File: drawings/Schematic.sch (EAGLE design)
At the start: 15 parts

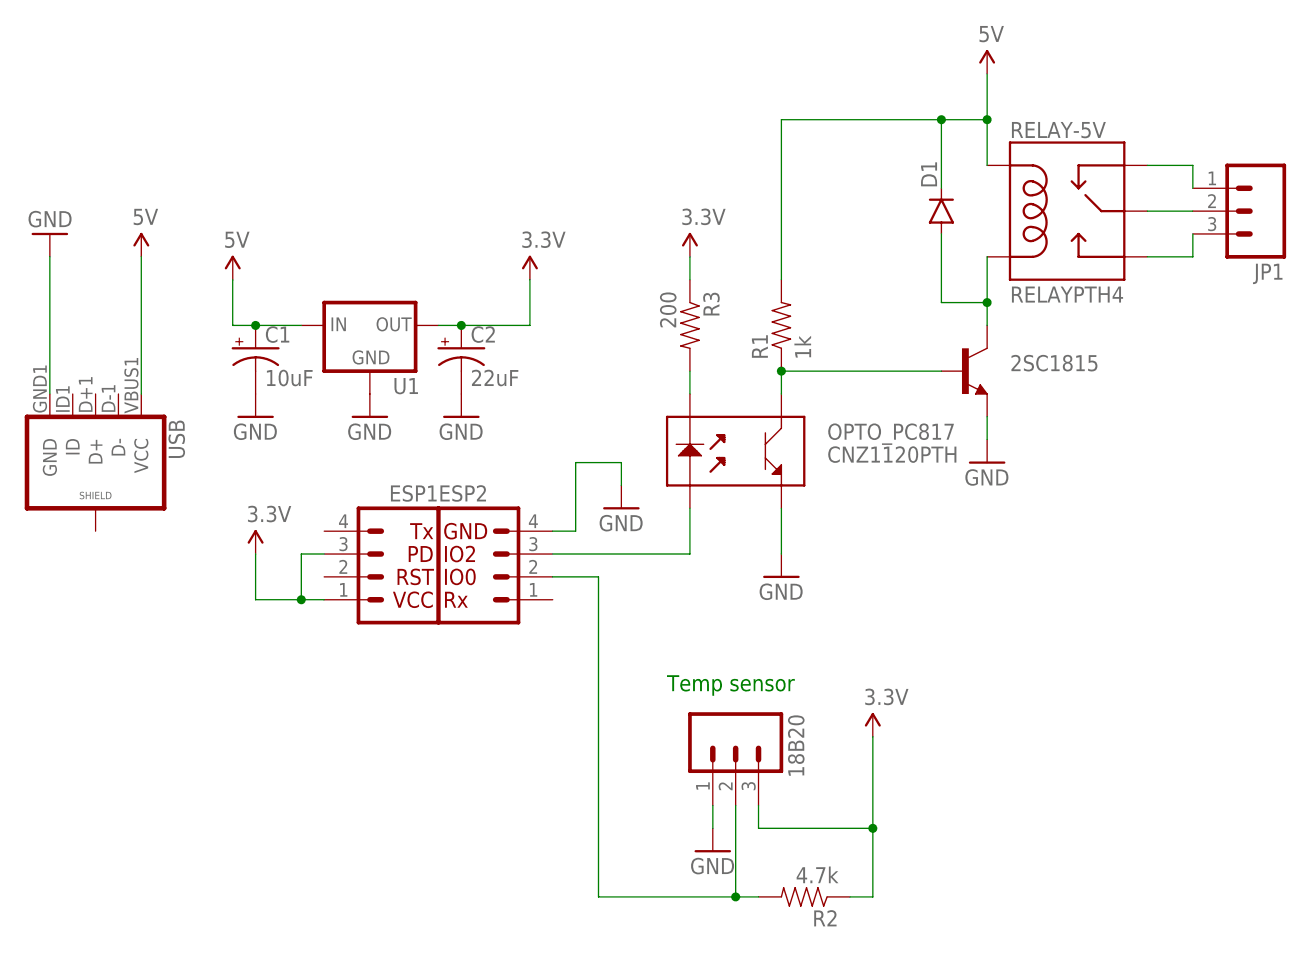
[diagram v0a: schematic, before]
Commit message: revise drawings
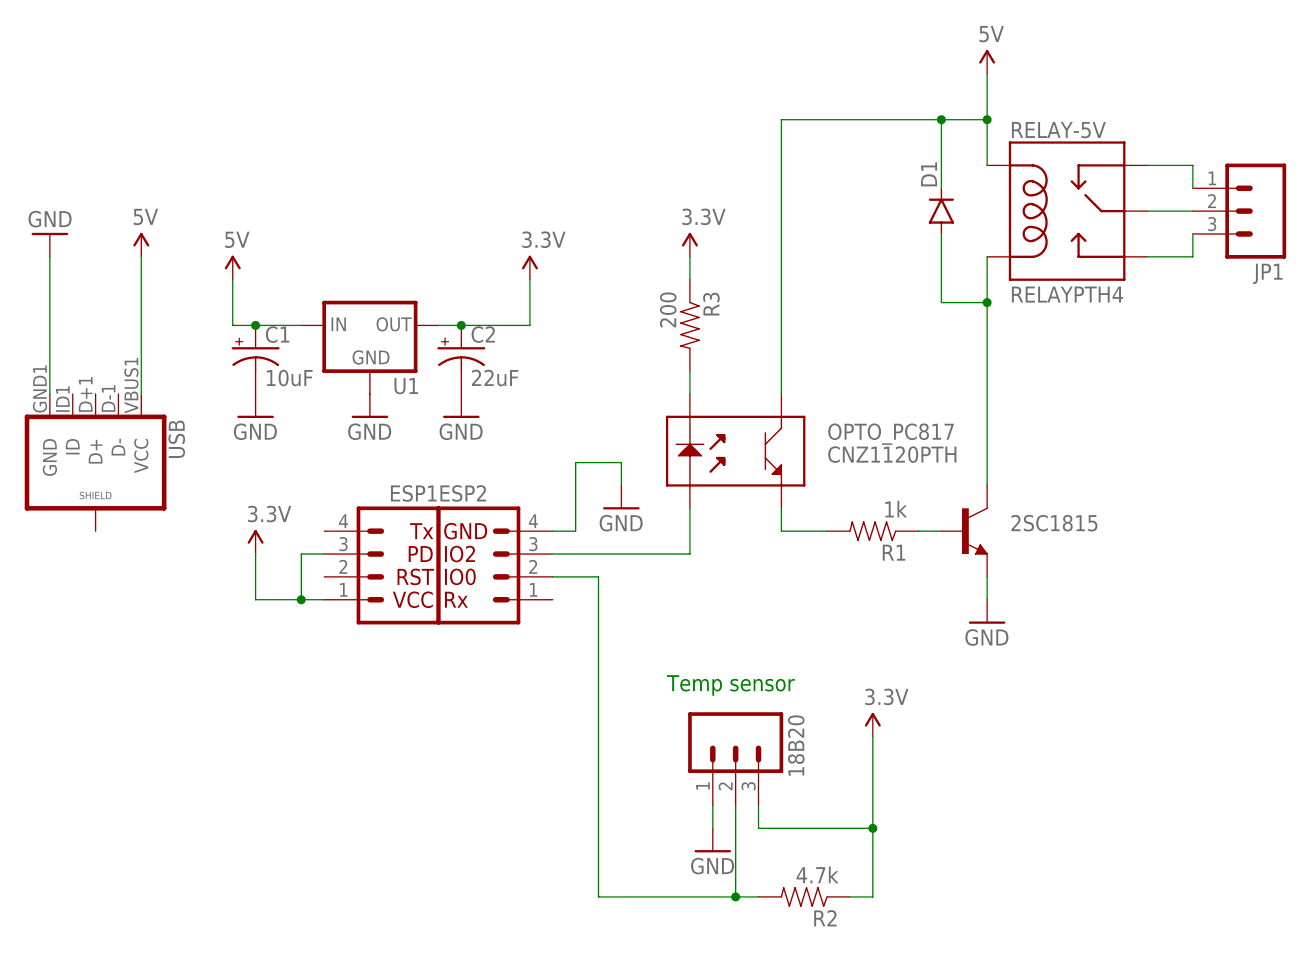
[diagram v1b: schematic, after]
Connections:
- new net N$9: 2SC1815.B, R1.1
- net 5V: now also OPTO_PC817.3; no longer R1.2
- net GND: no longer OPTO_PC817.4
- net N$1: now also OPTO_PC817.4, R1.2; no longer 2SC1815.B, OPTO_PC817.3, R1.1
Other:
- moved on the sheet: 2SC1815, R1
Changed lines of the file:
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@@
 <part name="R3" library="SparkFun-Resistors" deviceset="10KOHM-1/4W5%(PTH)" device="" value="200"/>
 <part name="SUPPLY8" library="SparkFun-Aesthetics" deviceset="3.3V" device=""/>
-<part name="GND7" library="SparkFun-Aesthetics" deviceset="GND" device=""/>
 <part name="JP1" library="ESP8266" deviceset="M03" device="1X03_NO_SILK"/>
 </parts>
@@
 <instance part="SUPPLY1" gate="G$1" x="17.78" y="38.1"/>
 <instance part="GND4" gate="1" x="58.42" y="43.18"/>
-<instance part="R1" gate="G$1" x="76.2" y="63.5" rot="R90"/>
-<instance part="2SC1815" gate="G$1" x="96.52" y="58.42"/>
+<instance part="R1" gate="G$1" x="86.36" y="40.64" rot="R180"/>
+<instance part="2SC1815" gate="G$1" x="96.52" y="40.64"/>
 <instance part="RELAY-5V" gate="G$1" x="109.22" y="76.2"/>
 <instance part="SUPPLY4" gate="G$1" x="99.06" y="91.44"/>
-<instance part="GND5" gate="1" x="99.06" y="48.26"/>
+<instance part="GND5" gate="1" x="99.06" y="30.48"/>
 <instance part="18B20" gate="G$1" x="71.12" y="17.78" rot="R270"/>
 <instance part="GND6" gate="1" x="68.58" y="5.08"/>
@@
 <instance part="R3" gate="G$1" x="66.04" y="63.5" rot="R270"/>
 <instance part="SUPPLY8" gate="G$1" x="66.04" y="71.12"/>
-<instance part="GND7" gate="1" x="76.2" y="35.56"/>
 <instance part="JP1" gate="G$1" x="129.54" y="76.2" rot="R180"/>
 </instances>
@@
 <wire x1="93.98" y1="86.36" x2="76.2" y2="86.36" width="0.1524" layer="91"/>
 <junction x="93.98" y="86.36"/>
-<pinref part="R1" gate="G$1" pin="2"/>
-<wire x1="76.2" y1="86.36" x2="76.2" y2="68.58" width="0.1524" layer="91"/>
+<pinref part="OPTO_PC817" gate="G$1" pin="3"/>
+<wire x1="76.2" y1="86.36" x2="76.2" y2="55.88" width="0.1524" layer="91"/>
 </segment>
 <segment>
@@
 </segment>
 <segment>
-<pinref part="2SC1815" gate="G$1" pin="E"/>
-<pinref part="GND5" gate="1" pin="GND"/>
-<wire x1="99.06" y1="53.34" x2="99.06" y2="50.8" width="0.1524" layer="91"/>
-</segment>
-<segment>
 <pinref part="18B20" gate="G$1" pin="1"/>
 <pinref part="GND6" gate="1" pin="GND"/>
@@
 </segment>
 <segment>
-<pinref part="OPTO_PC817" gate="G$1" pin="4"/>
-<pinref part="GND7" gate="1" pin="GND"/>
-<wire x1="76.2" y1="43.18" x2="76.2" y2="38.1" width="0.1524" layer="91"/>
-</segment>
-</net>
-<net name="N$1" class="0">
-<segment>
-<pinref part="R1" gate="G$1" pin="1"/>
-<pinref part="2SC1815" gate="G$1" pin="B"/>
-<wire x1="76.2" y1="58.42" x2="93.98" y2="58.42" width="0.1524" layer="91"/>
-<junction x="76.2" y="58.42"/>
-<pinref part="OPTO_PC817" gate="G$1" pin="3"/>
-<wire x1="76.2" y1="58.42" x2="76.2" y2="55.88" width="0.1524" layer="91"/>
+<pinref part="2SC1815" gate="G$1" pin="E"/>
+<pinref part="GND5" gate="1" pin="GND"/>
+<wire x1="99.06" y1="35.56" x2="99.06" y2="33.02" width="0.1524" layer="91"/>
 </segment>
 </net>
@@
 <wire x1="99.06" y1="71.12" x2="99.06" y2="66.04" width="0.1524" layer="91"/>
 <pinref part="D1" gate="G$1" pin="A"/>
-<wire x1="99.06" y1="66.04" x2="99.06" y2="63.5" width="0.1524" layer="91"/>
+<wire x1="99.06" y1="66.04" x2="99.06" y2="45.72" width="0.1524" layer="91"/>
 <wire x1="93.98" y1="73.66" x2="93.98" y2="66.04" width="0.1524" layer="91"/>
 <wire x1="93.98" y1="66.04" x2="99.06" y2="66.04" width="0.1524" layer="91"/>
@@
 </segment>
 </net>
+<net name="N$1" class="0">
+<segment>
+<pinref part="OPTO_PC817" gate="G$1" pin="4"/>
+<wire x1="76.2" y1="43.18" x2="76.2" y2="40.64" width="0.1524" layer="91"/>
+<pinref part="R1" gate="G$1" pin="2"/>
+<wire x1="76.2" y1="40.64" x2="81.28" y2="40.64" width="0.1524" layer="91"/>
+</segment>
+</net>
+<net name="N$9" class="0">
+<segment>
+<pinref part="R1" gate="G$1" pin="1"/>
+<pinref part="2SC1815" gate="G$1" pin="B"/>
+<wire x1="91.44" y1="40.64" x2="93.98" y2="40.64" width="0.1524" layer="91"/>
+</segment>
+</net>
